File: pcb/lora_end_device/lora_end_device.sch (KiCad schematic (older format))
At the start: 34 parts, among them J1 USB_B_Micro, J2 UFL, J3 SMA, J4 UART, J5 Reset, J6 PRG, J7 Sensor, U2 MCP6021, U3 LD1117, U4 RFM95W, U5 ESP-12S

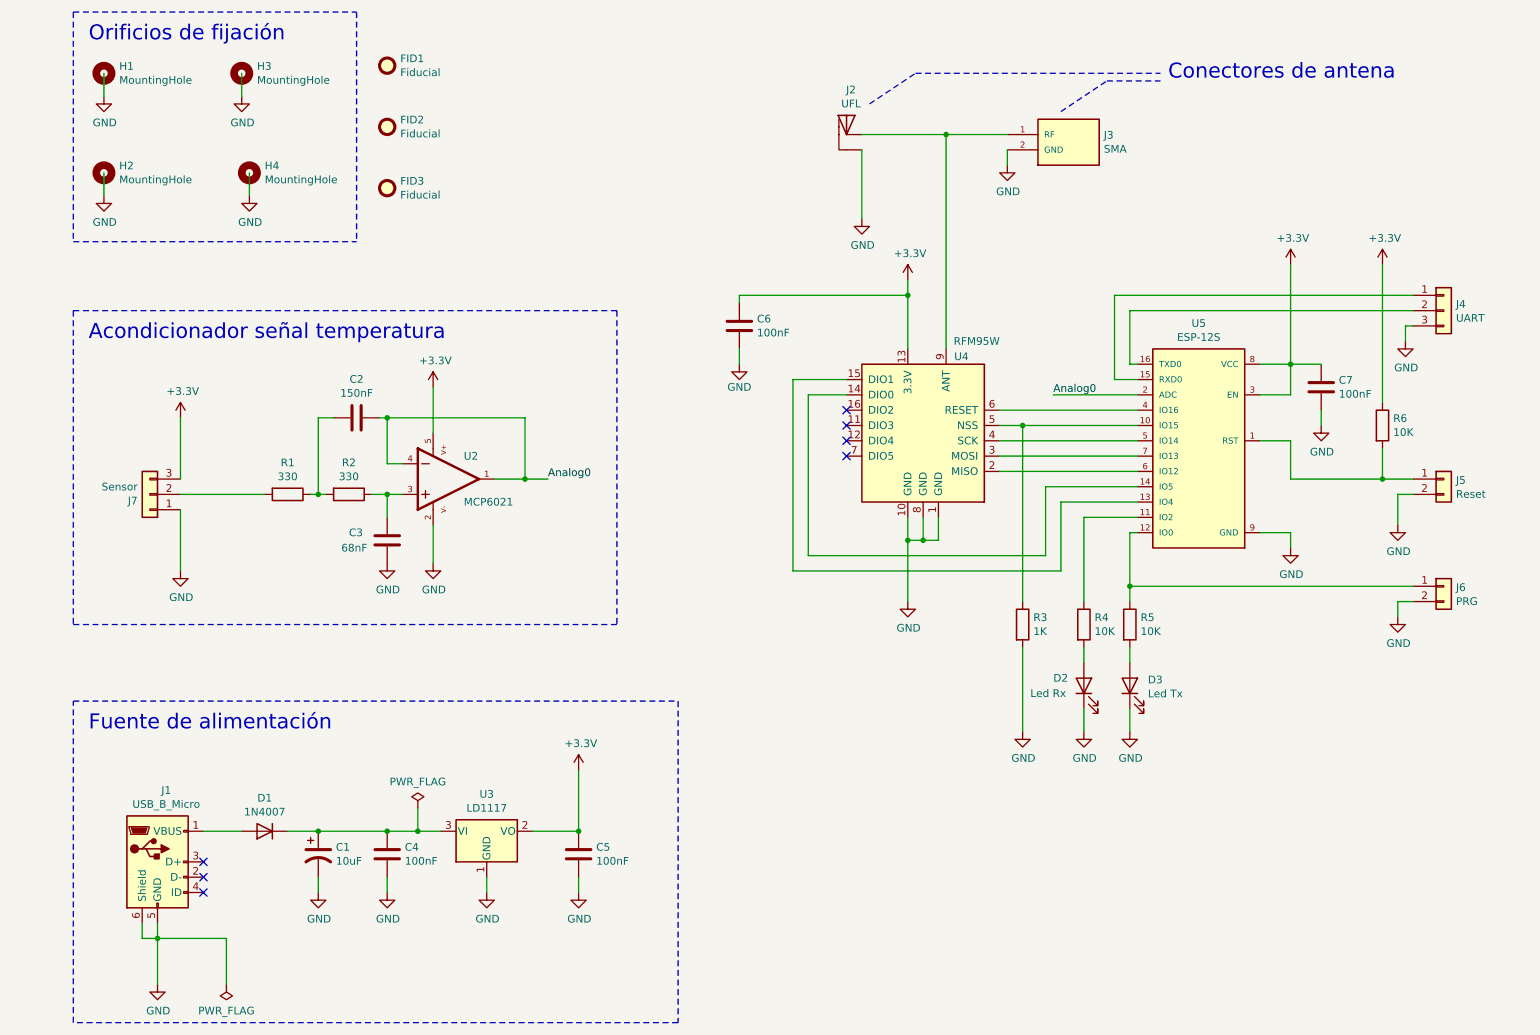
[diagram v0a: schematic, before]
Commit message: add ruteo
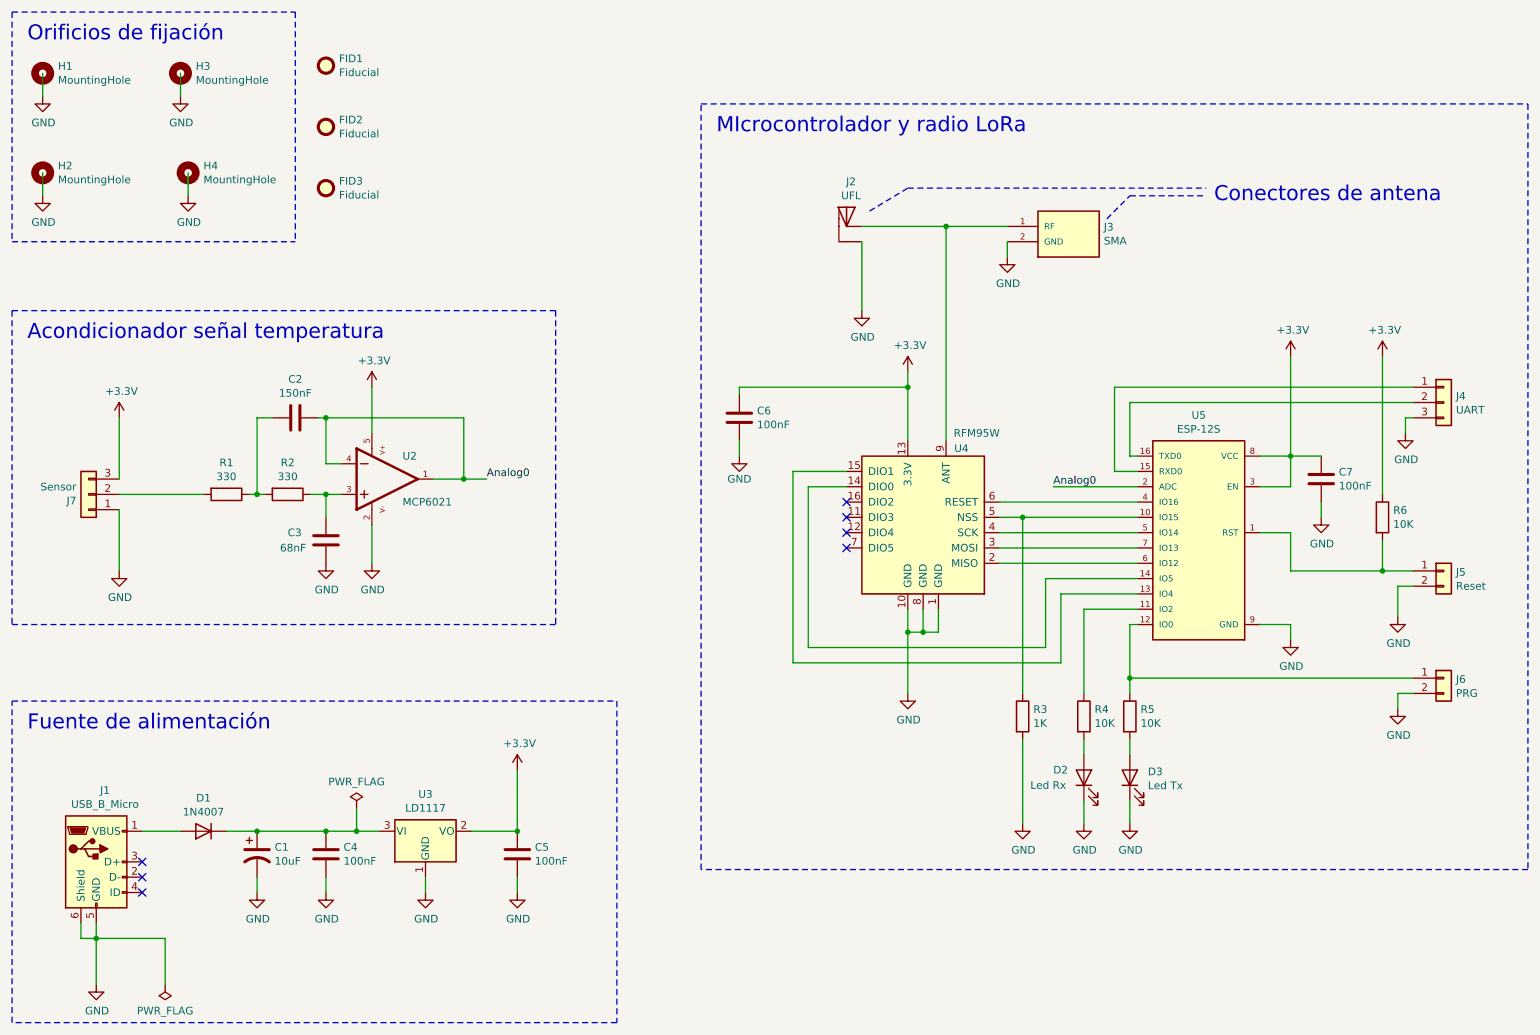
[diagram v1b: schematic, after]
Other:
- note added: "MIcrocontrolador y radio LoRa"
- moved on the sheet: C1, C2, C3, C4, C5, C6, C7, D1, D2, D3, FID1, FID2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
